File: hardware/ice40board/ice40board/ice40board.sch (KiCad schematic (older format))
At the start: 8 parts, among them P1 Power, P2 Analog, P3 Digital, P4 Digital, P5 CONN_01X01, P6 CONN_01X01, P7 CONN_01X01, P8 CONN_01X01

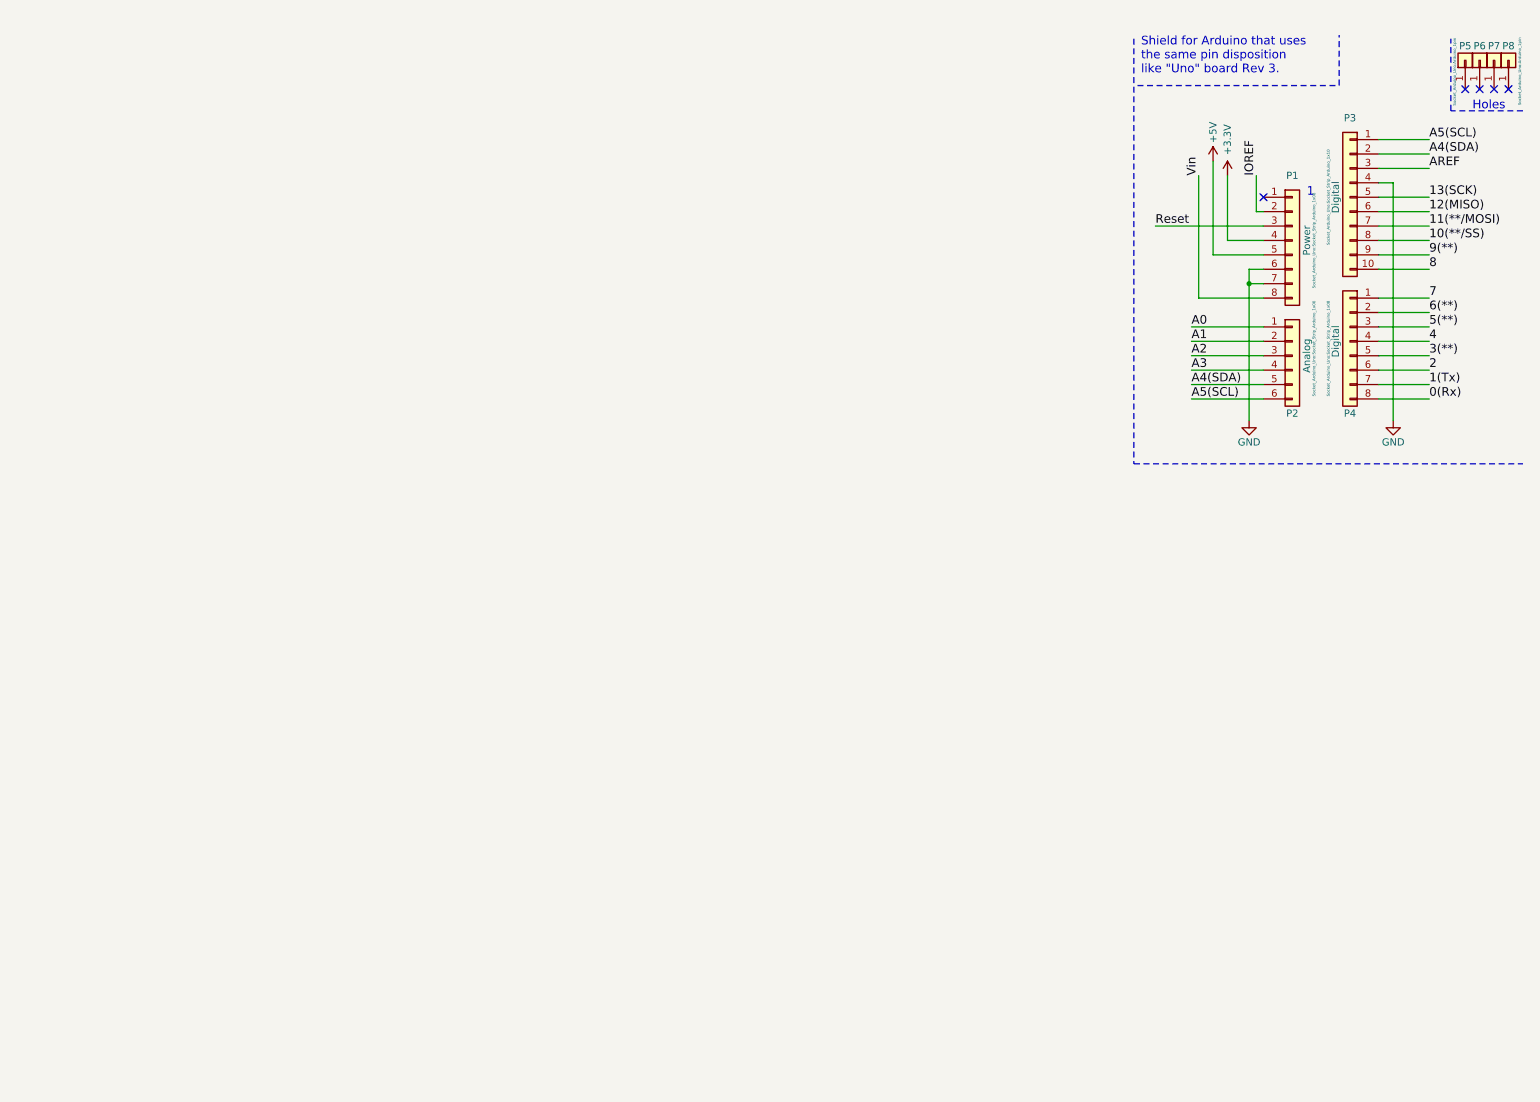
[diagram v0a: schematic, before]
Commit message: ice40 board
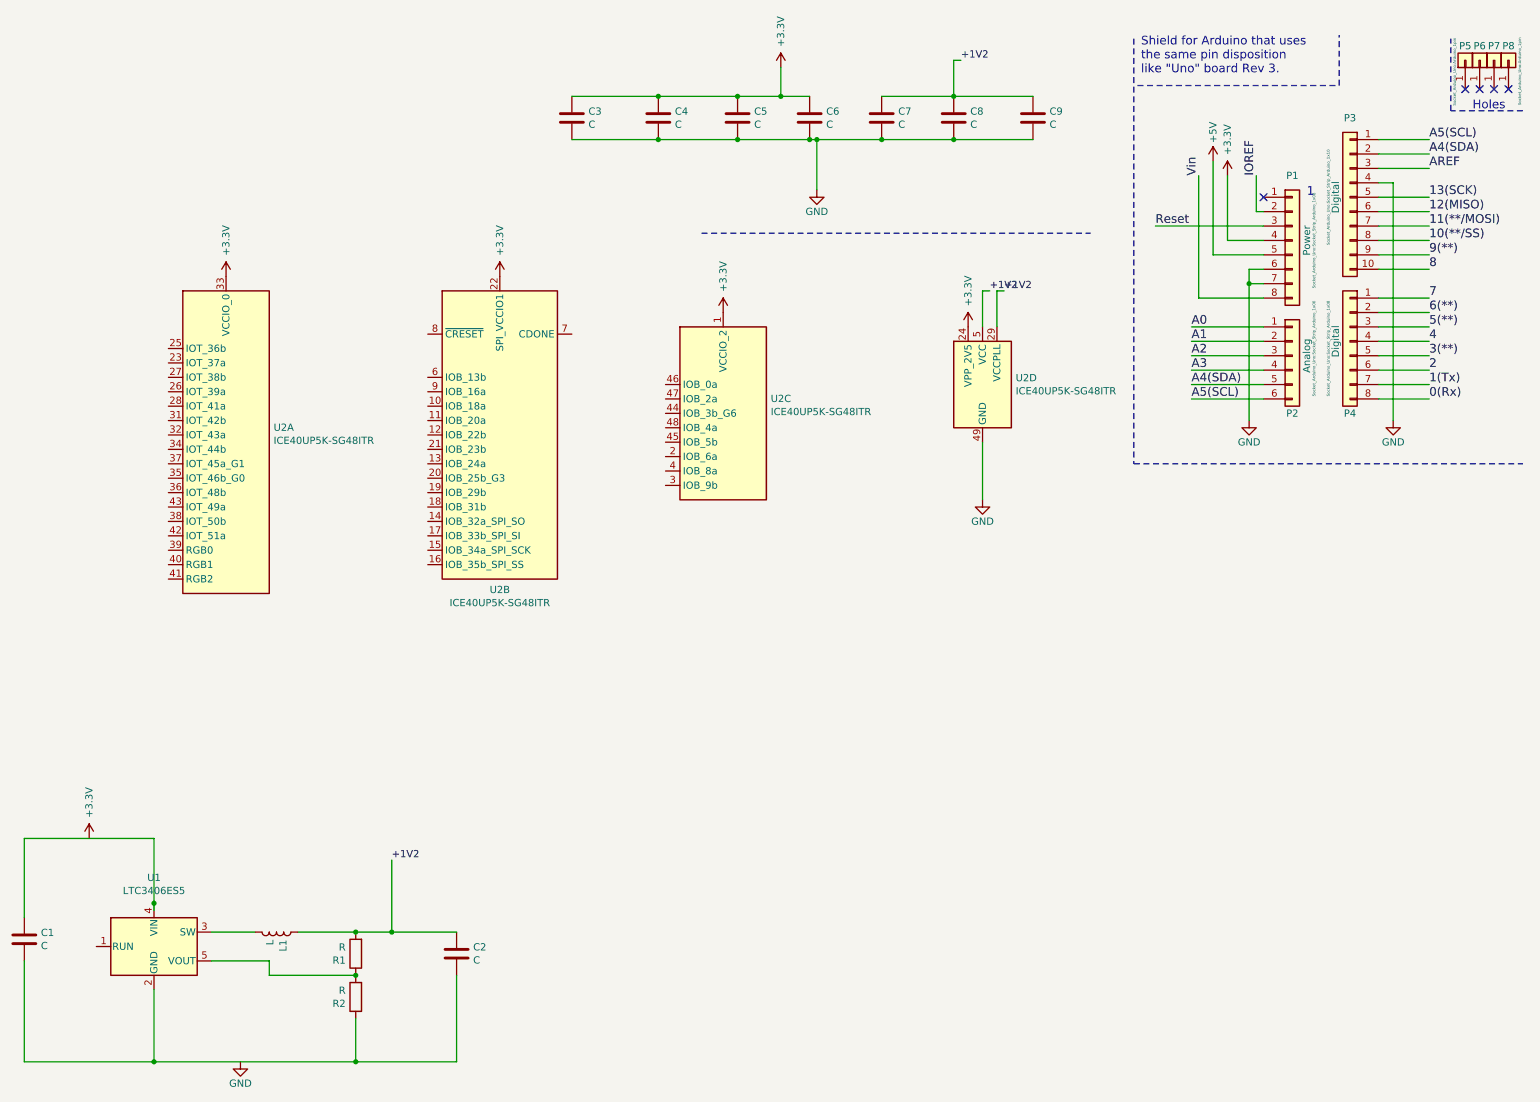
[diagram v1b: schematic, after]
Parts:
- added C1, C2, C3, C4, C5, C6, C7, C8, C9: C, symbol Device:C
- added L1: L, symbol Device:L
- added R1, R2: R, symbol Device:R
- added U1: LTC3406ES5, Package_TO_SOT_SMD:TSOT-23-5, symbol Regulator_Switching:LTC3406ES5
- added U2: ICE40UP5K-SG48ITR, Package_DFN_QFN:QFN-48-1EP_7x7mm_P0.5mm_EP5.6x5.6mm, symbol FPGA_Lattice:ICE40UP5K-SG48ITR
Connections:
- net +3V3: now also C3.1, C4.1, C5.1, C6.1, U2.1 (VCCIO_2), U2.22 (SPI_VCCIO1), U2.24 (VPP_2V5), U2.33 (VCCIO_0)
- net GND: now also C3.2, C4.2, C5.2, C6.2, C7.2, C8.2, C9.2, U2.49 (GND)
- new net: C1.2, C2.2, R2.1, U1.2 (GND)
- new net: L1.2, U1.3 (SW)
- new net: C1.1, U1.4 (VIN)
- new net: R1.1, R2.2, U1.5 (VOUT)
- new net +1V2: C2.1, C7.1, C8.1, C9.1, L1.1, R1.2, U2.29 (VCCPLL), U2.30 (VCC), U2.5 (VCC)
